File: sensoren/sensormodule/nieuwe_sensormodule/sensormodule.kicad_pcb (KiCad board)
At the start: 2 copper layers, 12 parts, among them J1 Screw_Terminal_01x05, U1 TCRT5000, U2 TCRT5000, U3 TCRT5000

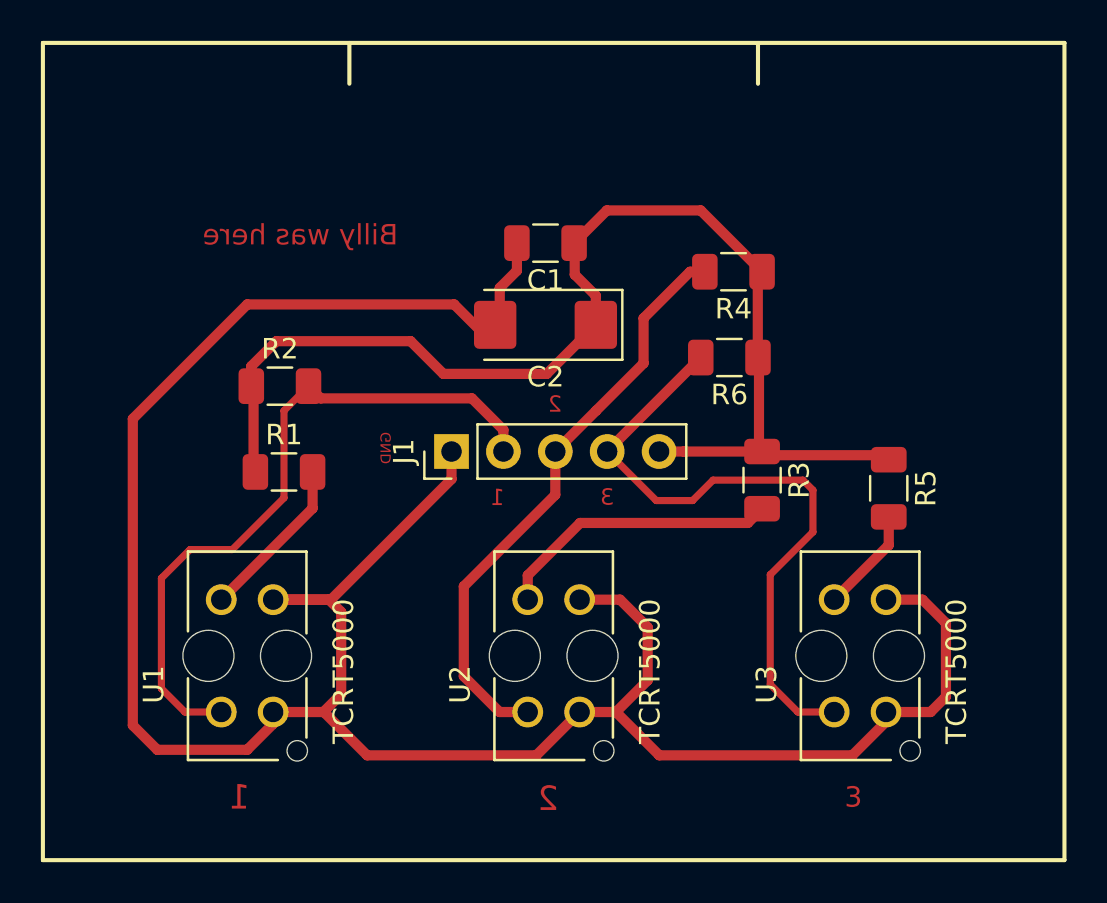
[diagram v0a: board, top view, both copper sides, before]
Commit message: update
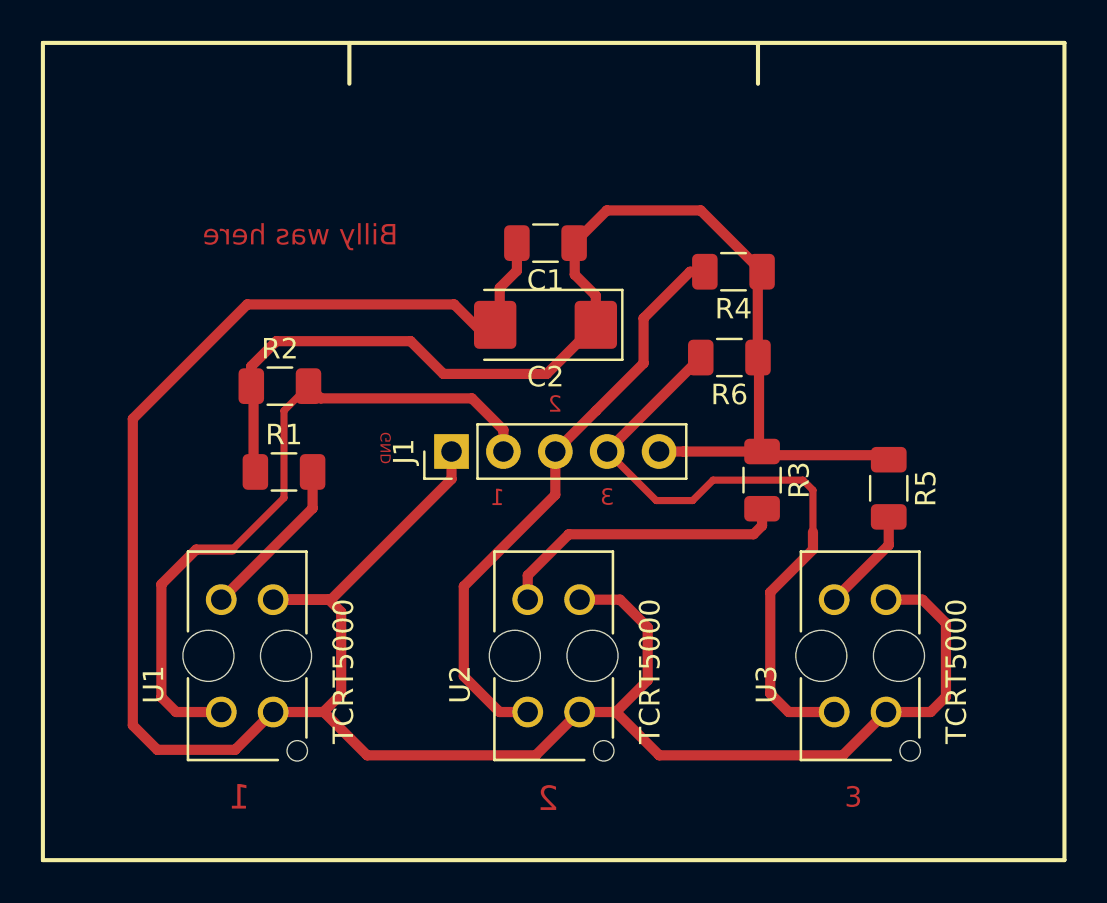
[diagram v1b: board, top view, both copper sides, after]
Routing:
- net GND: track 122.9 -> 122.3 mm
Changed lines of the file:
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@@
     (thickness 1.6)
     (drawings 16)
-    (tracks 108)
+    (tracks 110)
     (zones 0)
     (modules 12)
@@
   )
   (setup
-    (last_trace_width 0.25)
+    (last_trace_width 0.5)
     (user_trace_width 0.35)
     (user_trace_width 0.5)
@@
   (segment (start 109.1 57.25) (end 115 51.35) (width 0.5) (layer F.Cu) (net 2))
   (segment (start 106.27 57.25) (end 109.1 57.25) (width 0.5) (layer F.Cu) (net 2))
-  (segment (start 125.17 64.87) (end 123.05 62.75) (width 0.5) (layer F.Cu) (net 2))
-  (segment (start 134.62 64.87) (end 125.17 64.87) (width 0.5) (layer F.Cu) (net 2))
-  (segment (start 136.27 62.75) (end 136.27 63.22) (width 0.5) (layer F.Cu) (net 2))
-  (segment (start 136.27 63.22) (end 134.62 64.87) (width 0.5) (layer F.Cu) (net 2))
   (segment (start 108.69 62.75) (end 106.27 62.75) (width 0.5) (layer F.Cu) (net 2))
-  (segment (start 119.15 64.87) (end 121.27 62.75) (width 0.5) (layer F.Cu) (net 2))
-  (segment (start 109 57.25) (end 109.6 57.85) (width 0.5) (layer F.Cu) (net 2))
-  (segment (start 106.27 57.25) (end 109 57.25) (width 0.5) (layer F.Cu) (net 2))
-  (segment (start 109.6 57.85) (end 109.6 61.88) (width 0.5) (layer F.Cu) (net 2))
-  (segment (start 108.74 62.74) (end 110.87 64.87) (width 0.5) (layer F.Cu) (net 2))
-  (segment (start 109.6 61.88) (end 108.74 62.74) (width 0.5) (layer F.Cu) (net 2))
-  (segment (start 110.87 64.87) (end 119.15 64.87) (width 0.5) (layer F.Cu) (net 2))
-  (segment (start 105 64.6) (end 106.27 63.33) (width 0.5) (layer F.Cu) (net 2))
-  (segment (start 100.6 64.6) (end 105 64.6) (width 0.5) (layer F.Cu) (net 2))
-  (segment (start 106.27 63.33) (end 106.27 62.75) (width 0.5) (layer F.Cu) (net 2))
-  (segment (start 99.4 63.4) (end 100.6 64.6) (width 0.5) (layer F.Cu) (net 2))
-  (segment (start 116.67 44.2675) (end 116.67 44.34) (width 0.5) (layer F.Cu) (net 2))
-  (segment (start 116.67 44.34) (end 115.13 42.8) (width 0.5) (layer F.Cu) (net 2))
-  (segment (start 115.13 42.8) (end 105 42.8) (width 0.5) (layer F.Cu) (net 2))
-  (segment (start 105 42.8) (end 99.4 48.4) (width 0.5) (layer F.Cu) (net 2))
-  (segment (start 117.1375 43.8) (end 116.67 44.2675) (width 0.5) (layer F.Cu) (net 2))
-  (segment (start 99.4 48.4) (end 99.4 63.4) (width 0.5) (layer F.Cu) (net 2))
   (segment (start 117.36 43.5775) (end 117.1375 43.8) (width 0.5) (layer F.Cu) (net 2))
   (segment (start 117.36 41.99) (end 117.36 43.5775) (width 0.5) (layer F.Cu) (net 2))
   (segment (start 118.2 39.8) (end 118.2 41.15) (width 0.5) (layer F.Cu) (net 2))
   (segment (start 118.2 41.15) (end 117.36 41.99) (width 0.5) (layer F.Cu) (net 2))
+  (segment (start 106.26 62.75) (end 106.27 62.75) (width 0.5) (layer F.Cu) (net 2))
+  (segment (start 104.41 64.6) (end 106.26 62.75) (width 0.5) (layer F.Cu) (net 2))
+  (segment (start 100.6 64.6) (end 104.41 64.6) (width 0.5) (layer F.Cu) (net 2))
+  (segment (start 99.4 63.4) (end 100.6 64.6) (width 0.5) (layer F.Cu) (net 2))
+  (segment (start 116.67 44.2675) (end 116.67 44.34) (width 0.5) (layer F.Cu) (net 2))
+  (segment (start 117.1375 43.8) (end 116.67 44.2675) (width 0.5) (layer F.Cu) (net 2))
+  (segment (start 116.67 44.34) (end 115.13 42.8) (width 0.5) (layer F.Cu) (net 2))
+  (segment (start 105 42.8) (end 99.4 48.4) (width 0.5) (layer F.Cu) (net 2))
+  (segment (start 115.13 42.8) (end 105 42.8) (width 0.5) (layer F.Cu) (net 2))
+  (segment (start 99.4 48.4) (end 99.4 63.4) (width 0.5) (layer F.Cu) (net 2))
+  (segment (start 125.17 64.87) (end 123.05 62.75) (width 0.5) (layer F.Cu) (net 2))
+  (segment (start 136.27 62.75) (end 134.15 64.87) (width 0.5) (layer F.Cu) (net 2))
+  (segment (start 134.15 64.87) (end 125.17 64.87) (width 0.5) (layer F.Cu) (net 2))
+  (segment (start 109 57.25) (end 109.6 57.85) (width 0.5) (layer F.Cu) (net 2))
+  (segment (start 106.27 57.25) (end 109 57.25) (width 0.5) (layer F.Cu) (net 2))
+  (segment (start 109.6 57.85) (end 109.6 61.88) (width 0.5) (layer F.Cu) (net 2))
+  (segment (start 109.6 61.88) (end 108.74 62.74) (width 0.5) (layer F.Cu) (net 2))
+  (segment (start 119.12 64.87) (end 121.24 62.75) (width 0.5) (layer F.Cu) (net 2))
+  (segment (start 108.74 62.74) (end 110.87 64.87) (width 0.5) (layer F.Cu) (net 2))
+  (segment (start 121.24 62.75) (end 121.27 62.75) (width 0.5) (layer F.Cu) (net 2))
+  (segment (start 110.87 64.87) (end 119.12 64.87) (width 0.5) (layer F.Cu) (net 2))
   (segment (start 108.6 47.4) (end 108 46.8) (width 0.5) (layer F.Cu) (net 3))
   (segment (start 116 47.4) (end 108.6 47.4) (width 0.5) (layer F.Cu) (net 3))
   (segment (start 117.54 50) (end 117.54 48.94) (width 0.5) (layer F.Cu) (net 3))
   (segment (start 117.54 48.94) (end 116 47.4) (width 0.5) (layer F.Cu) (net 3))
-  (segment (start 101.95 62.75) (end 103.73 62.75) (width 0.35) (layer F.Cu) (net 3))
   (segment (start 106.8 48) (end 106.8 52.27) (width 0.35) (layer F.Cu) (net 3))
   (segment (start 108 46.8) (end 106.8 48) (width 0.35) (layer F.Cu) (net 3))
-  (segment (start 100.8 61.6) (end 101.95 62.75) (width 0.35) (layer F.Cu) (net 3))
   (segment (start 106.8 52.27) (end 104.27 54.8) (width 0.35) (layer F.Cu) (net 3))
-  (segment (start 104.27 54.8) (end 102.2 54.8) (width 0.35) (layer F.Cu) (net 3))
-  (segment (start 102.2 54.8) (end 100.8 56.2) (width 0.35) (layer F.Cu) (net 3))
-  (segment (start 100.8 56.2) (end 100.8 61.6) (width 0.35) (layer F.Cu) (net 3))
+  (segment (start 101.52 62.75) (end 103.73 62.75) (width 0.5) (layer F.Cu) (net 3))
+  (segment (start 100.8 62.03) (end 101.52 62.75) (width 0.5) (layer F.Cu) (net 3))
+  (segment (start 100.8 56.5) (end 100.8 62.03) (width 0.5) (layer F.Cu) (net 3))
+  (segment (start 104.27 54.8) (end 102.5 54.8) (width 0.5) (layer F.Cu) (net 3))
+  (segment (start 102.5 54.8) (end 100.8 56.5) (width 0.5) (layer F.Cu) (net 3))
   (segment (start 118.73 62.75) (end 117.35 62.75) (width 0.5) (layer F.Cu) (net 4))
   (segment (start 117.35 62.75) (end 115.6 61) (width 0.5) (layer F.Cu) (net 4))
@@
   (segment (start 126.8 52.4) (end 125.02 52.4) (width 0.35) (layer F.Cu) (net 5))
   (segment (start 127.8 51.4) (end 126.8 52.4) (width 0.35) (layer F.Cu) (net 5))
-  (segment (start 133.73 62.75) (end 131.95 62.75) (width 0.35) (layer F.Cu) (net 5))
-  (segment (start 130.6 61.4) (end 130.6 56.03) (width 0.35) (layer F.Cu) (net 5))
   (segment (start 132.2 51.4) (end 127.8 51.4) (width 0.35) (layer F.Cu) (net 5))
-  (segment (start 130.6 56.03) (end 132.69 53.94) (width 0.35) (layer F.Cu) (net 5))
   (segment (start 132.69 53.94) (end 132.69 51.89) (width 0.35) (layer F.Cu) (net 5))
-  (segment (start 131.95 62.75) (end 130.6 61.4) (width 0.35) (layer F.Cu) (net 5))
   (segment (start 132.69 51.89) (end 132.2 51.4) (width 0.35) (layer F.Cu) (net 5))
+  (segment (start 132.69 54.8) (end 132.69 53.94) (width 0.5) (layer F.Cu) (net 5))
+  (segment (start 130.6 56.89) (end 132.69 54.8) (width 0.5) (layer F.Cu) (net 5))
+  (segment (start 130.6 61.85) (end 130.6 56.89) (width 0.5) (layer F.Cu) (net 5))
+  (segment (start 133.73 62.75) (end 131.5 62.75) (width 0.5) (layer F.Cu) (net 5))
+  (segment (start 131.5 62.75) (end 130.6 61.85) (width 0.5) (layer F.Cu) (net 5))
   (segment (start 108.2 52.78) (end 103.73 57.25) (width 0.5) (layer F.Cu) (net 6))
   (segment (start 108.2 51) (end 108.2 52.78) (width 0.5) (layer F.Cu) (net 6))
-  (segment (start 129.50429 53.49571) (end 121.29571 53.49571) (width 0.5) (layer F.Cu) (net 7))
-  (segment (start 130.2 52.8) (end 129.50429 53.49571) (width 0.5) (layer F.Cu) (net 7))
   (segment (start 118.73 56.06142) (end 118.73 57.25) (width 0.5) (layer F.Cu) (net 7))
-  (segment (start 121.29571 53.49571) (end 118.73 56.06142) (width 0.5) (layer F.Cu) (net 7))
+  (segment (start 120.74142 54.05) (end 118.73 56.06142) (width 0.5) (layer F.Cu) (net 7))
+  (segment (start 129.78 54.05) (end 120.74142 54.05) (width 0.5) (layer F.Cu) (net 7))
+  (segment (start 130.2 52.8) (end 130.2 53.63) (width 0.5) (layer F.Cu) (net 7))
+  (segment (start 130.2 53.63) (end 129.78 54.05) (width 0.5) (layer F.Cu) (net 7))
   (segment (start 136.4 54.58) (end 133.73 57.25) (width 0.5) (layer F.Cu) (net 8))
   (segment (start 136.4 53.2) (end 136.4 54.58) (width 0.5) (layer F.Cu) (net 8))
